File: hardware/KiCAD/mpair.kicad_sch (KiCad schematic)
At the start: 26 parts, among them J1 PJ-063AH, J2 PJ-063AH, J3 DX07S016JA1R1500, J4 ARJP11A-MASA-B-A-EMU2, U1 USBLC6-2SC6

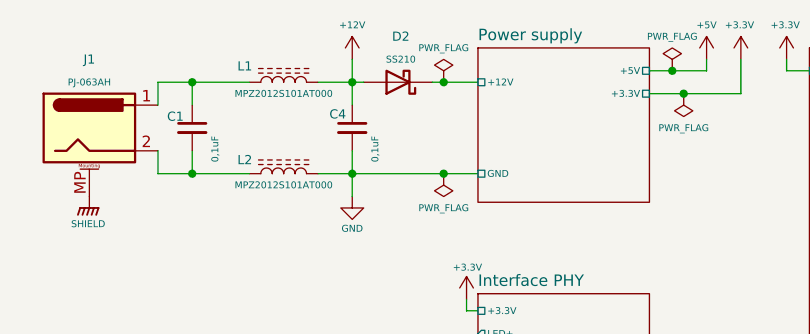
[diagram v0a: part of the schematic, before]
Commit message: update
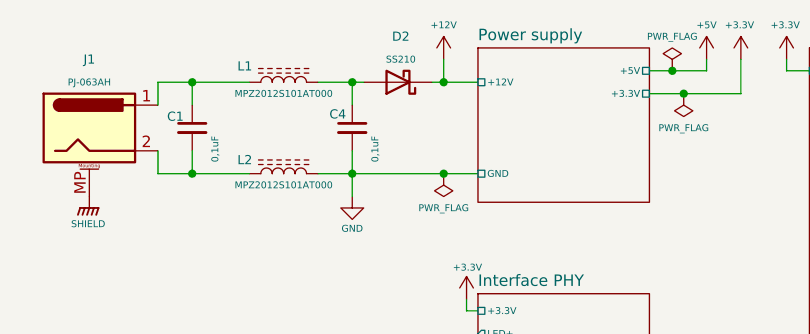
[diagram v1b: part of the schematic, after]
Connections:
- net Power supply/+12V is gone; now on net +12V: D2.1 (K)
- net +12V: no longer C4.1, D2.2 (A), L1.2
- new net: C4.1, D2.2 (A), L1.2
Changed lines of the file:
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@@
 	)
 	(junction
-		(at 73.66 25.4)
-		(diameter 0)
-		(color 0 0 0 0)
-	)
-	(junction
 		(at 73.66 101.6)
 		(diameter 0)
@@
 	)
 	(junction
+		(at 73.66 25.4)
+		(diameter 0)
+		(color 0 0 0 0)
+	)
+	(junction
 		(at 139.7 93.98)
 		(diameter 0)
@@
 	(wire
 		(pts
-			(xy 73.66 25.4) (xy 77.47 25.4)
-		)
-		(stroke
-			(width 0)
-			(type default)
-		)
-	)
-	(wire
-		(pts
 			(xy 40.64 91.44) (xy 40.64 93.98)
 		)
@@
 	(wire
 		(pts
+			(xy 73.66 25.4) (xy 77.47 25.4)
+		)
+		(stroke
+			(width 0)
+			(type default)
+		)
+	)
+	(wire
+		(pts
 			(xy 68.58 66.04) (xy 77.47 66.04)
 		)
@@
 	(wire
 		(pts
+			(xy 73.66 22.86) (xy 73.66 25.4)
+		)
+		(stroke
+			(width 0)
+			(type default)
+		)
+	)
+	(wire
+		(pts
 			(xy 96.52 100.33) (xy 101.6 100.33)
 		)
@@
 	(wire
 		(pts
-			(xy 63.5 22.86) (xy 63.5 25.4)
-		)
-		(stroke
-			(width 0)
-			(type default)
-		)
-	)
-	(wire
-		(pts
 			(xy 172.72 59.69) (xy 175.26 59.69)
 		)
@@
 	)
 	(symbol
-		(lib_id "power:PWR_FLAG")
-		(at 73.66 25.4 0)
-		(unit 1)
-		(exclude_from_sim no)
-		(in_bom yes)
-		(on_board yes)
-		(dnp no)
-		(fields_autoplaced yes)
-		(property "Reference" "#FLG03"
-			(at 73.66 23.495 0)
-			(effects
-				(font
-					(size 1.27 1.27)
-				)
-				(hide yes)
-			)
-		)
-		(property "Value" "PWR_FLAG"
-			(at 73.66 21.59 0)
-			(effects
-				(font
-					(size 0.762 0.762)
-				)
-			)
-		)
-		(property "Footprint" ""
-			(at 73.66 25.4 0)
-			(effects
-				(font
-					(size 1.27 1.27)
-				)
-				(hide yes)
-			)
-		)
-		(property "Datasheet" "~"
-			(at 73.66 25.4 0)
-			(effects
-				(font
-					(size 1.27 1.27)
-				)
-				(hide yes)
-			)
-		)
-		(property "Description" "Special symbol for telling ERC where power comes from"
-			(at 73.66 25.4 0)
-			(effects
-				(font
-					(size 1.27 1.27)
-				)
-				(hide yes)
-			)
-		)
-		(pin "1"
-		)
-		(instances
-			(project ""
-				(path "/c7dbdcbe-6da7-4d67-a2bd-18f9bca31cdc"
-					(reference "#FLG03")
-					(unit 1)
-				)
-			)
-		)
-	)
-	(symbol
 		(lib_id "power:+3.3V")
 		(at 153.67 78.74 0)
@@
 	(symbol
 		(lib_id "power:+3.3V")
-		(at 63.5 22.86 0)
+		(at 73.66 22.86 0)
 		(unit 1)
 		(exclude_from_sim no)
@@
 		(fields_autoplaced yes)
 		(property "Reference" "#PWR05"
-			(at 63.5 26.67 0)
+			(at 73.66 26.67 0)
 			(effects
 				(font
@@
 		)
 		(property "Value" "+12V"
-			(at 63.5 19.05 0)
+			(at 73.66 19.05 0)
 			(effects
 				(font
@@
 		)
 		(property "Footprint" ""
-			(at 63.5 22.86 0)
+			(at 73.66 22.86 0)
 			(effects
 				(font
@@
 		)
 		(property "Datasheet" ""
-			(at 63.5 22.86 0)
+			(at 73.66 22.86 0)
 			(effects
 				(font
@@
 		)
 		(property "Description" "Power symbol creates a global label with name \"+3.3V\""
-			(at 63.5 22.86 0)
+			(at 73.66 22.86 0)
 			(effects
 				(font
